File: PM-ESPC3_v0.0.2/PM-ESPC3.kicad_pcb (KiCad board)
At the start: 2 copper layers, 39.8 x 99.8 mm, 34 parts, among them J1 U254-051T-4BH83-S1S, J2 AFA07-S10FCC-00, J3 R-RJ11R04P-A802, J4 R-RJ11R04P-A802, J5 AFA07-S10FCC-00, J6 AFA07-S10FCC-00, J8 AFA07-S10FCC-00, SW1 Button, SW2 Button, SW4 DIP 3 pos, U1 ESP32-C3-WROOM-02U-N4, U2 CJA1117B-3.3, U3 MAX3485

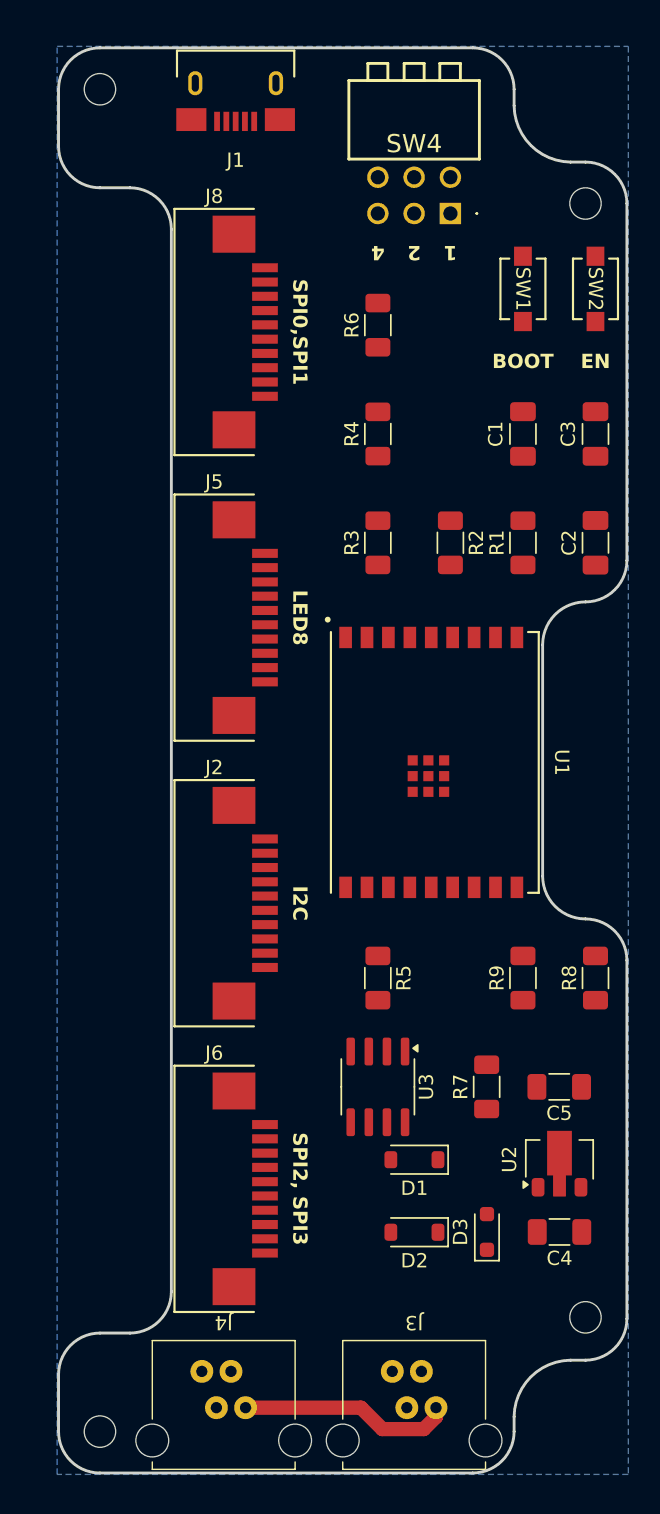
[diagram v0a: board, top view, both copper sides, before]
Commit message: PM-Debug
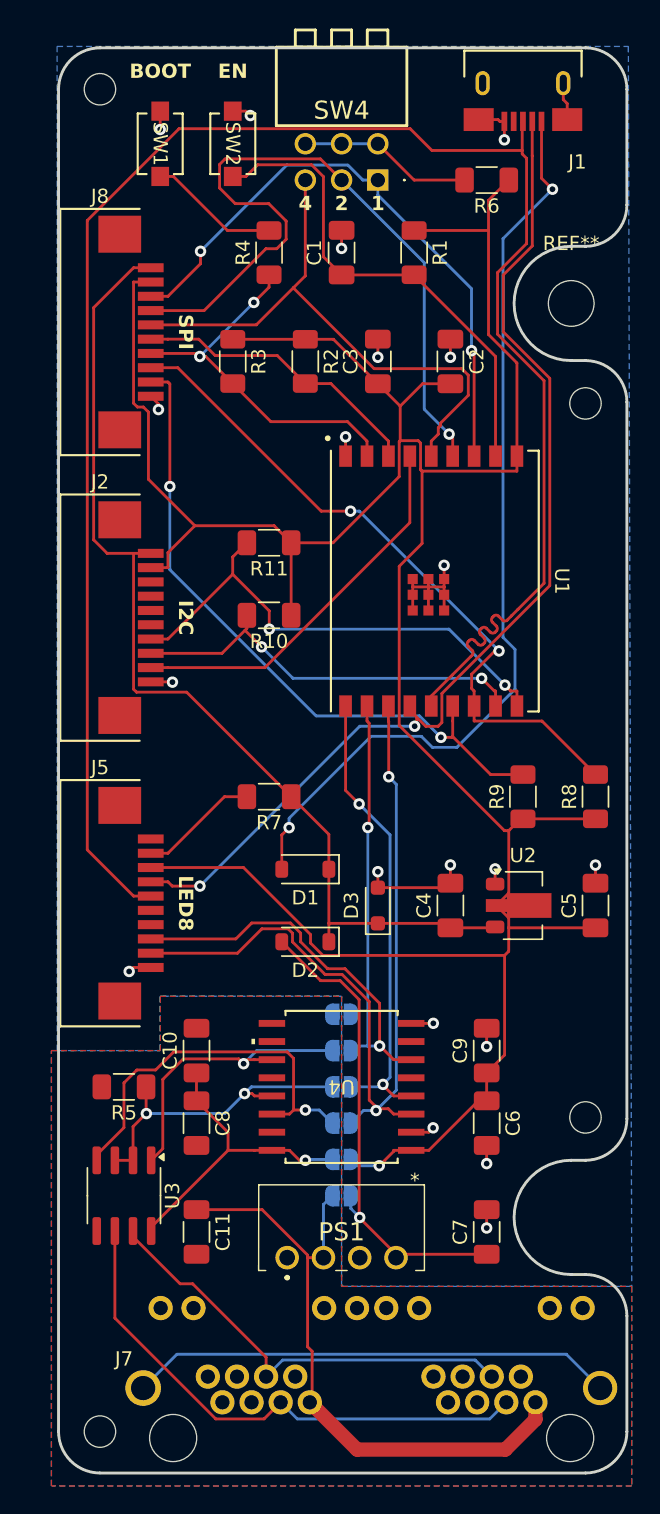
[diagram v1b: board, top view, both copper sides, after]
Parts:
- removed J3, J4: R-RJ11R04P-A802, kicad_inventree_lib:R-RJ11R04P-A802
- removed J6: AFA07-S10FCC-00, kicad_inventree_lib:CONN10_AFA07-S10_JUS
- added C10: 10uF, Capacitor_SMD:C_1206_3216Metric_Pad1.33x1.80mm_HandSolder, F.Cu at (59.8, 120.3)
- added C11: 10uF, Capacitor_SMD:C_1206_3216Metric_Pad1.33x1.80mm_HandSolder, F.Cu at (59.8, 133.0)
- added C6: 100nF, Capacitor_SMD:C_1206_3216Metric_Pad1.33x1.80mm_HandSolder, F.Cu at (80.1, 125.4)
- added C7: 10uF, Capacitor_SMD:C_1206_3216Metric_Pad1.33x1.80mm_HandSolder, F.Cu at (80.1, 133.0)
- added C8: 100nF, Capacitor_SMD:C_1206_3216Metric_Pad1.33x1.80mm_HandSolder, F.Cu at (59.8, 125.4)
- added C9: 10uF, Capacitor_SMD:C_1206_3216Metric_Pad1.33x1.80mm_HandSolder, F.Cu at (80.1, 120.3)
- added J7: ~, kicad_inventree_lib:HC-WK88-H16-1X2-DB, F.Cu at (67.7, 139.9)
- added JP1: SolderJumper_2_Open, Jumper:SolderJumper-2_P1.3mm_Open_RoundedPad1.0x1.5mm, B.Cu at (69.9, 125.4)
- added JP2: SolderJumper_2_Open, Jumper:SolderJumper-2_P1.3mm_Open_RoundedPad1.0x1.5mm, B.Cu at (69.9, 120.3)
- added JP3: SolderJumper_2_Open, Jumper:SolderJumper-2_P1.3mm_Open_RoundedPad1.0x1.5mm, B.Cu at (69.9, 122.9)
- added JP4: SolderJumper_2_Open, Jumper:SolderJumper-2_P1.3mm_Open_RoundedPad1.0x1.5mm, B.Cu at (69.9, 127.9)
- added JP5: SolderJumper_2_Open, Jumper:SolderJumper-2_P1.3mm_Open_RoundedPad1.0x1.5mm, B.Cu at (69.9, 117.8)
- added JP6: SolderJumper_2_Open, Jumper:SolderJumper-2_P1.3mm_Open_RoundedPad1.0x1.5mm, B.Cu at (69.9, 130.5)
- added PS1: B0505S-1WR3, kicad_inventree_lib:B0505S1WR3, F.Cu at (66.1, 134.8)
- added R10: 3k3, Resistor_SMD:R_1206_3216Metric_Pad1.30x1.75mm_HandSolder, F.Cu at (64.8, 89.8)
- added R11: 3k3, Resistor_SMD:R_1206_3216Metric_Pad1.30x1.75mm_HandSolder, F.Cu at (64.8, 84.8)
- added REF**: MountingHole_3.2mm_M3, MountingHole:MountingHole_3.2mm_M3, F.Cu at (86.0, 68.0)
- added U4: CA-IS3641HW, kicad_inventree_lib:SOIC16-WBW_CLG-M, F.Cu at (69.9, 122.9)
- moved SW1 27.4 mm to (57.2, 56.8)
- moved SW2 27.4 mm to (62.3, 56.8)
- moved R7 25.4 mm to (64.8, 102.5), turned to 180 degrees
- moved C4 24.1 mm to (77.5, 110.2), turned to 90 degrees
- moved D3 24.1 mm to (72.5, 110.2)
- moved D1 21.7 mm to (67.4, 107.6)
- moved D2 21.7 mm to (67.4, 112.7)
- moved R1 21.7 mm to (75.0, 64.4), turned to -90 degrees
- moved J2 21.5 mm to (53.0, 90.0)
- moved J5 21.5 mm to (53.0, 110.0)
- moved J1 20.1 mm to (83.9, 55.4)
- moved R5 19.3 mm to (54.7, 122.9), turned to 180 degrees
- moved U3 19.3 mm to (54.7, 130.5)
- moved U2 18.0 mm to (82.6, 110.2), turned to 0 degrees
- moved C1 18.0 mm to (69.9, 64.4)
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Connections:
- D2 pad 2: Net-(D2-A) -> +5V_BUS
- J5 pad 4: /LED0 -> /USB_D-
- J5 pad 5: /LED1 -> /USB_D+
- J5 pad 6: /LED2 -> unconnected-(J5-Pin_6-Pad6)
- J5 pad 7: /LED3 -> unconnected-(J5-Pin_7-Pad7)
- J5 pad 8: unconnected-(J5-Pin_8-Pad8) -> /UART_RX
- J5 pad 9: unconnected-(J5-Pin_9-Pad9) -> /UART_TX
- J8 pad 3: unconnected-(J8-Pin_3-Pad3) -> /MOSI
- J8 pad 4: /MOSI -> /MISO
- J8 pad 5: /MISO -> /SCK
- J8 pad 6: /SCK -> /CS0
- J8 pad 7: /CS0 -> /CS1
- J8 pad 8: /CS1 -> /CS2
- J8 pad 9: /INT -> /CS3
- R5 pad 1: /UART_DIR -> /UART_DIR_ISO
- R5 pad 2: GND -> GND_ISO
- SW4 pad 1: /SCK -> /MOSI
- SW4 pad 2: /MOSI -> /MISO
- SW4 pad 3: /LED0 -> /SCK
- U3 pad 1: /UART_RX -> /UART_RX_ISO
- U3 pad 2: /UART_DIR -> /UART_DIR_ISO
- U3 pad 3: /UART_DIR -> /UART_DIR_ISO
- U3 pad 4: /UART_TX -> /UART_TX_ISO
- U3 pad 5: GND -> GND_ISO
- U3 pad 8: +3.3V -> +3.3V_ISO
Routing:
- net +3.3V: track 0.00 -> 208.2 mm, vias 0 -> 1
- net /USB_D+: track 0.00 -> 134.0 mm
- net /USB_D-: track 0.00 -> 74.5 mm, vias 0 -> 2
- net +5V: track 0.00 -> 72.5 mm
- net Net-(D1-A): track 0.00 -> 65.9 mm, vias 0 -> 2
- net /UART_TX: track 0.00 -> 60.2 mm, vias 0 -> 2
- net /MISO: track 0.00 -> 52.0 mm, vias 0 -> 1
- net /UART_RX: track 0.00 -> 50.8 mm, vias 0 -> 2
- net /CS2: track 0.00 -> 48.6 mm, vias 0 -> 2
- net /CS3: track 0.00 -> 47.3 mm, vias 0 -> 2
- net GND: track 0.00 -> 44.7 mm, vias 0 -> 20
- net +5V_ISO: track 0.00 -> 44.6 mm
- net /MOSI: track 0.00 -> 42.8 mm, vias 0 -> 2
- net /SCK: track 0.00 -> 40.5 mm
- net /A: track 0.00 -> 37.9 mm
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- added copper zone on B.Cu, net GND_ISO
- added copper zone on F.Cu, net GND_ISO
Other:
- outline, holes or cut-outs redrawn
- board text added: "SPI"
- board text removed: "SPI0,SPI1"
- board text removed: "SPI2, SPI3"

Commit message: main
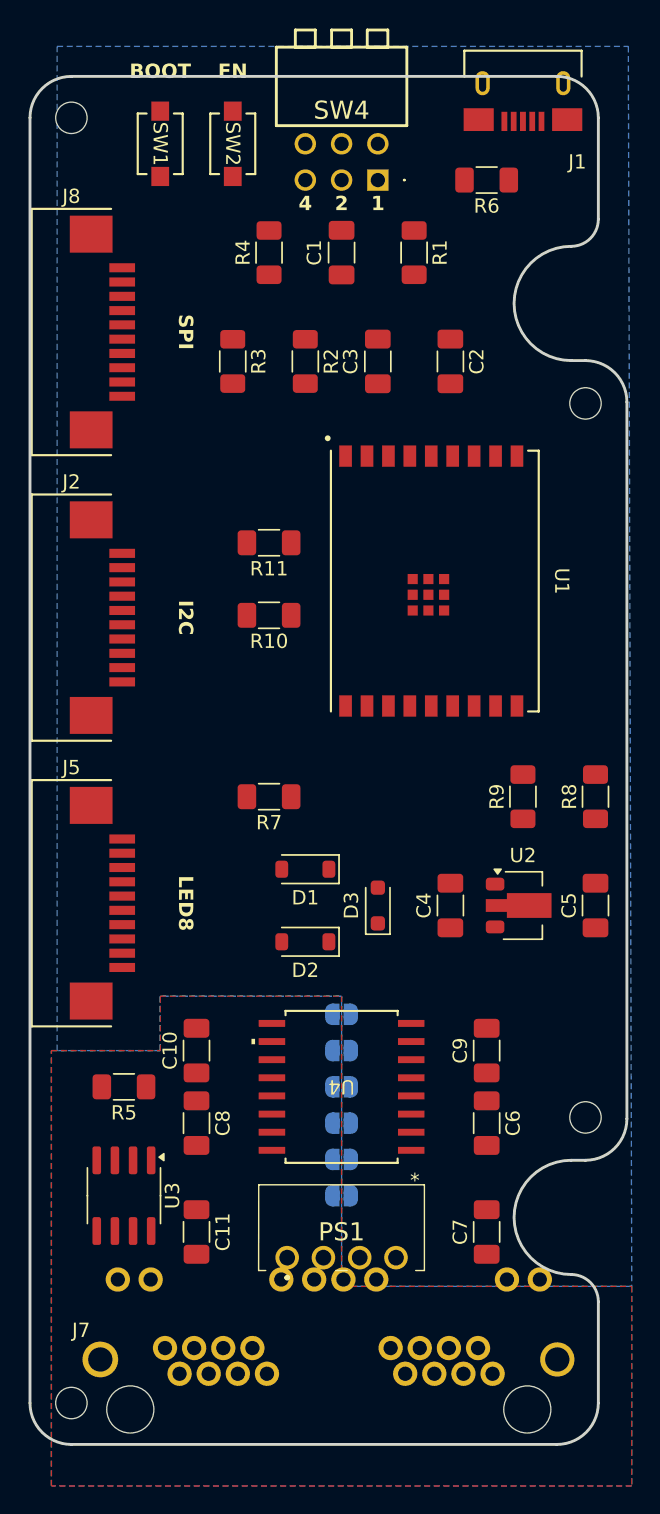
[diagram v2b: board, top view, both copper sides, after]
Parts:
- removed REF**: MountingHole_3.2mm_M3, MountingHole:MountingHole_3.2mm_M3
- moved J7 3.61 mm to (64.7, 137.9)
- moved H2 2.83 mm to (51.0, 145.0)
- moved H4 2.83 mm to (51.0, 55.0)
- moved J2 2.00 mm to (51.0, 90.0)
- moved J5 2.00 mm to (51.0, 110.0)
- moved J8 2.00 mm to (51.0, 70.0)
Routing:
- net +3.3V: track 208.2 -> 0.00 mm, vias 1 -> 0
- net /USB_D+: track 134.0 -> 0.00 mm
- net /USB_D-: track 74.5 -> 0.00 mm, vias 2 -> 0
- net +5V: track 72.5 -> 0.00 mm
- net Net-(D1-A): track 65.9 -> 0.00 mm, vias 2 -> 0
- net /UART_TX: track 60.2 -> 0.00 mm, vias 2 -> 0
- net /MISO: track 52.0 -> 0.00 mm, vias 1 -> 0
- net /UART_RX: track 50.8 -> 0.00 mm, vias 2 -> 0
- net /CS2: track 48.6 -> 0.00 mm, vias 2 -> 0
- net /CS3: track 47.3 -> 0.00 mm, vias 2 -> 0
- net GND: track 44.7 -> 0.00 mm, vias 20 -> 0
- net +5V_ISO: track 44.6 -> 0.00 mm
- net /MOSI: track 42.8 -> 0.00 mm, vias 2 -> 0
- net /SCK: track 40.5 -> 0.00 mm
- net /A: track 37.9 -> 0.00 mm
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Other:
- board size 39.8 x 99.8 mm -> 41.8 x 95.8 mm
